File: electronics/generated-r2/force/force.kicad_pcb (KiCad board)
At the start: 2 copper layers, 18 x 12 mm, 7 parts, among them J1 HALL_3V3_GND_OUT, U1 DRV5055A3QDBZR

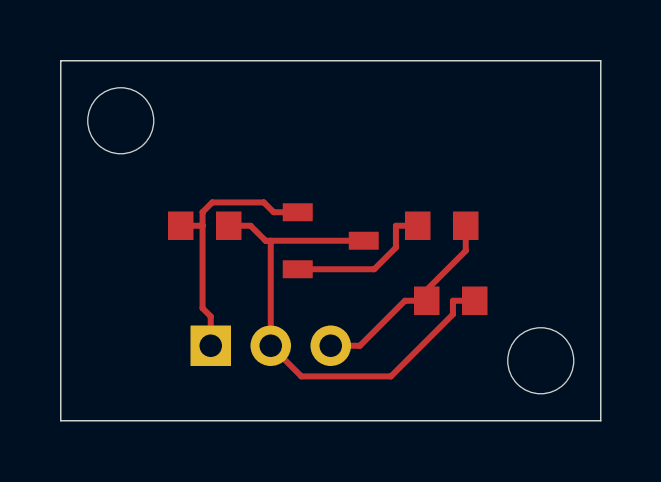
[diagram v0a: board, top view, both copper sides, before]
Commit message: build(r2): publish four routed boards and checks [skip ci]
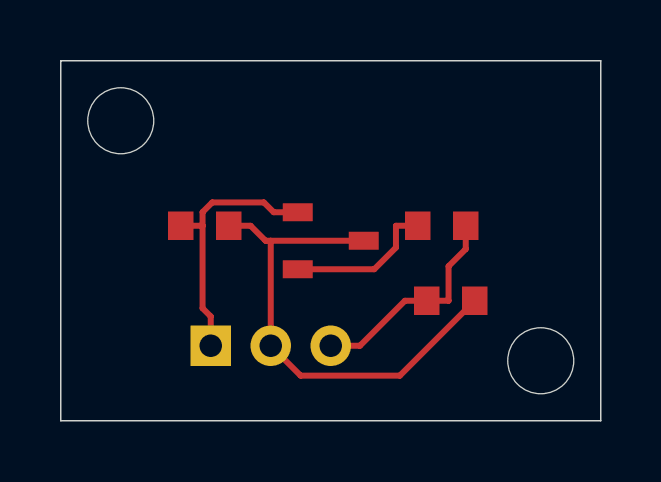
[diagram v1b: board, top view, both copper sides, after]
